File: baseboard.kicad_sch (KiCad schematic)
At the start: 27 parts, among them J10 AS7265X, J11 Conn_02x20_Odd_Even, J12 TFTLCD, J5 Screw_Terminal_01x02, J6 DCMI_CAMERA, J7 LCD_CHAR, J8 Conn_01x03, J9 Conn_01x03, U2 LM2676S-5, U3 AMS1117-3.3

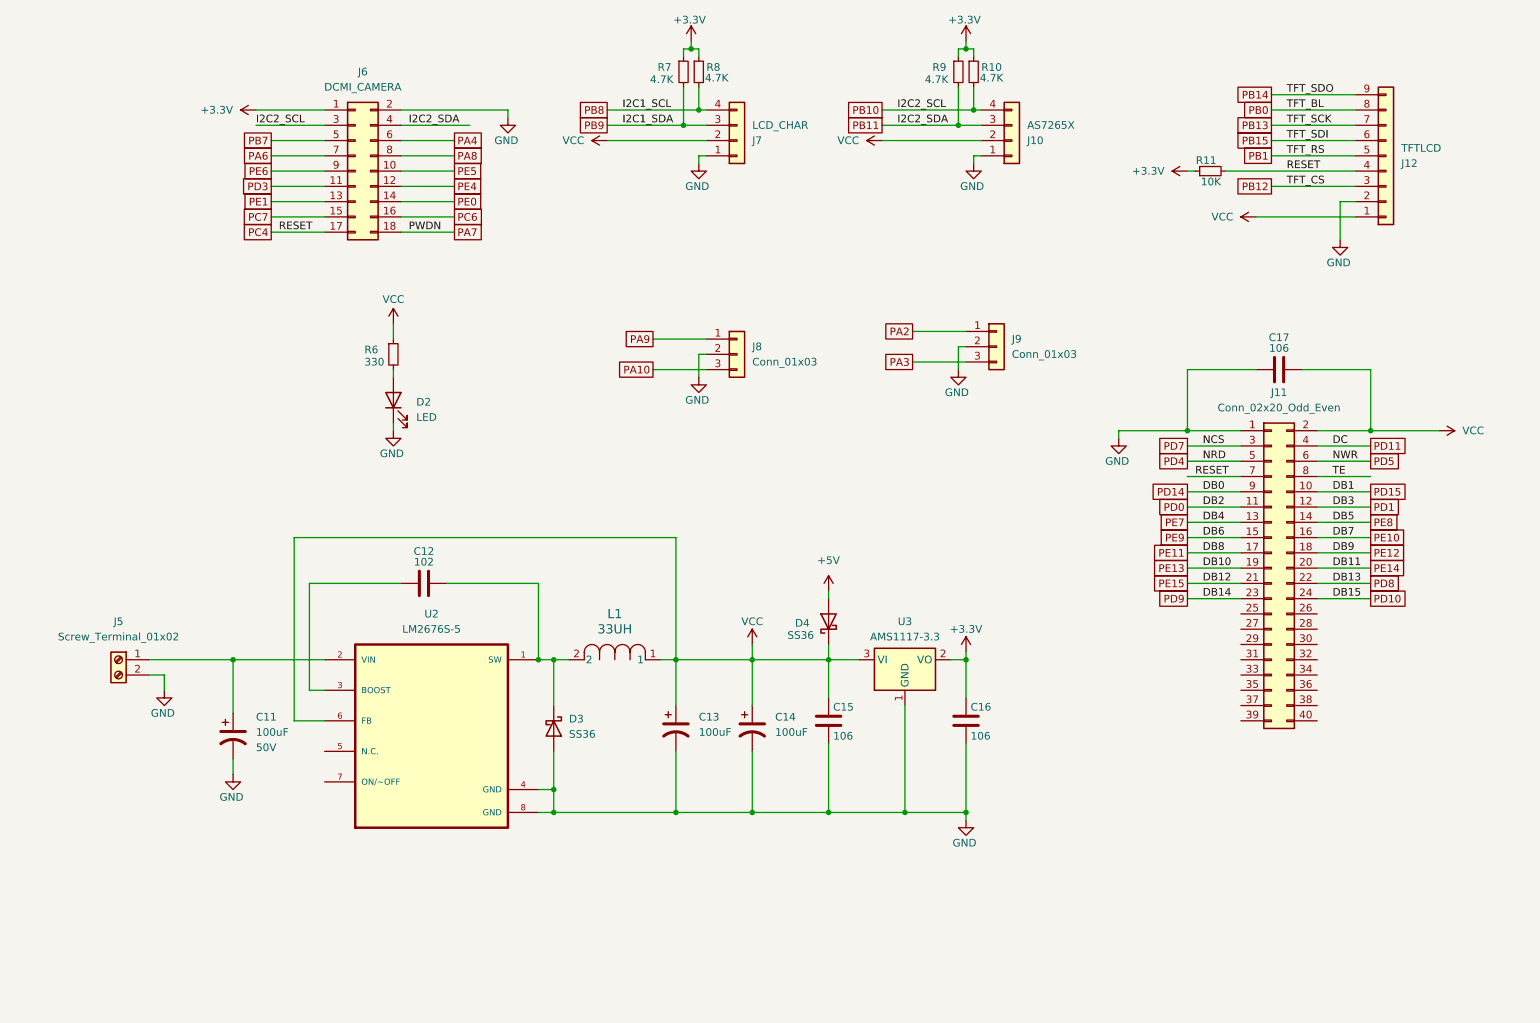
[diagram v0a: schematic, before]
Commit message: snapshot
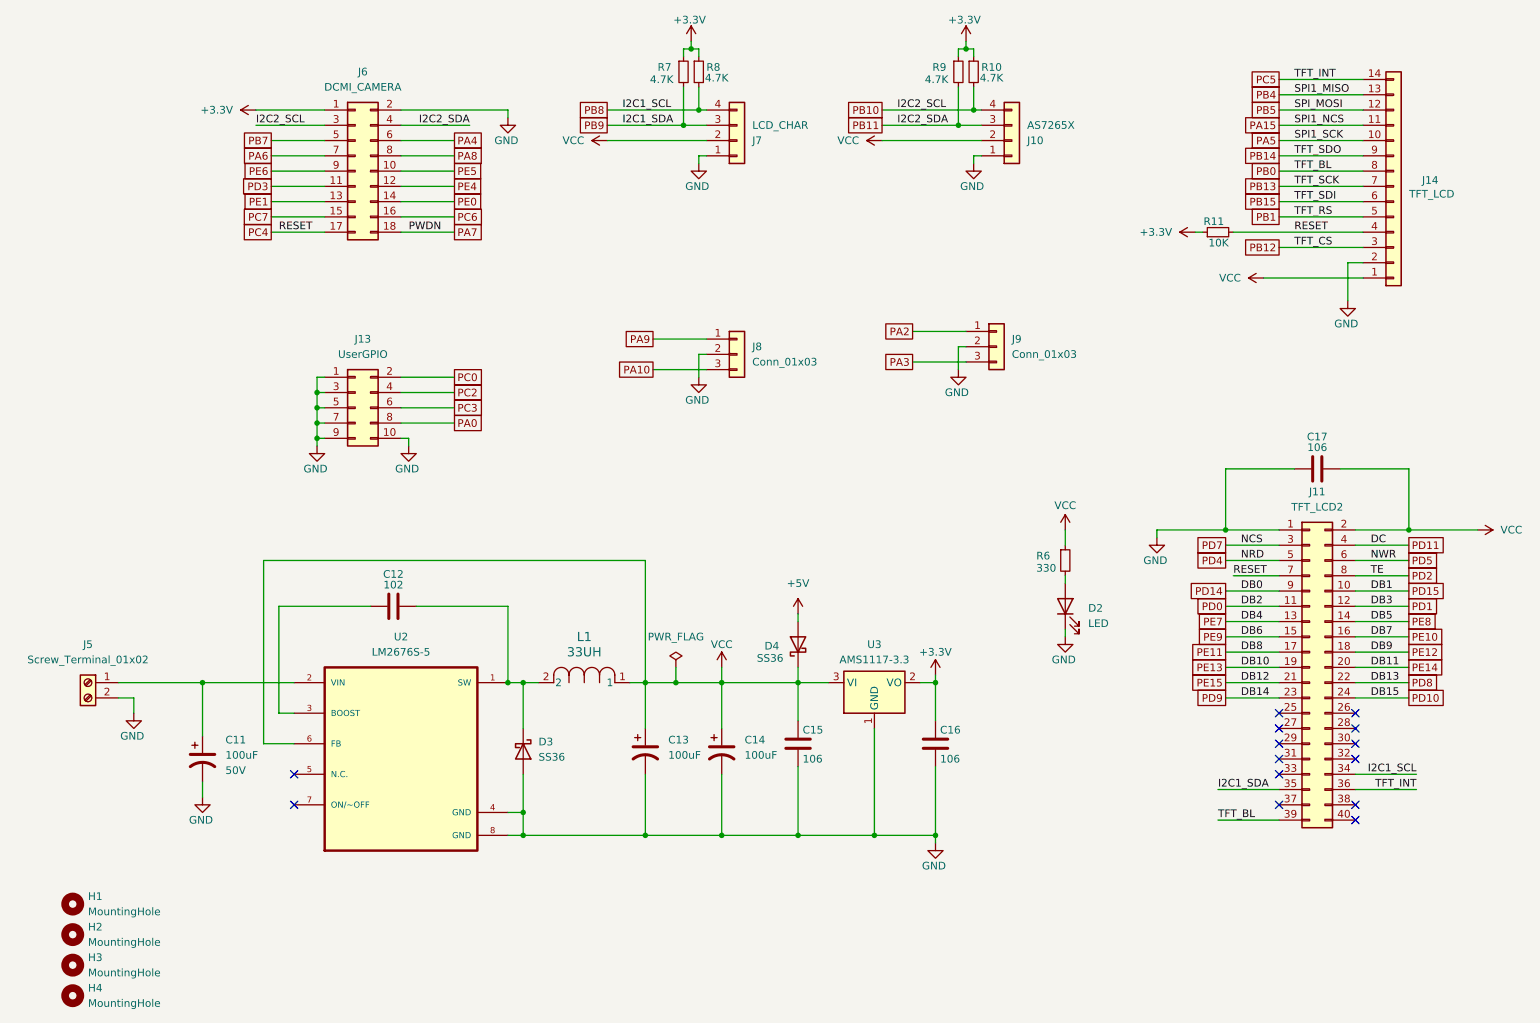
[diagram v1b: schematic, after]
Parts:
- removed J12: TFTLCD, Connector_PinHeader_2.54mm:PinHeader_1x09_P2.54mm_Vertical, symbol Connector_Generic:Conn_01x09
- added H1, H2, H3, H4: MountingHole, MountingHole:MountingHole_3.2mm_M3, symbol Mechanical:MountingHole
- added J13: UserGPIO, Connector_PinHeader_2.54mm:PinHeader_2x05_P2.54mm_Vertical, symbol Connector_Generic:Conn_02x05_Odd_Even
- added J14: TFT_LCD, Connector_PinHeader_2.54mm:PinHeader_1x14_P2.54mm_Vertical, symbol Connector_Generic:Conn_01x14
- J11: value Conn_02x20_Odd_Even -> TFT_LCD2
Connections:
- net GND: now also J13.1 (Pin_1), J13.10 (Pin_10), J13.3 (Pin_3), J13.5 (Pin_5), J13.7 (Pin_7), J13.9 (Pin_9), J14.2 (Pin_2)
- net PB0: now also J11.39 (Pin_39), J14.8 (Pin_8)
- net PB1: now also J14.5 (Pin_5)
- net PB12: now also J14.3 (Pin_3)
- net PB13: now also J14.7 (Pin_7)
- net PB14: now also J14.9 (Pin_9)
- net PB15: now also J14.6 (Pin_6)
- net PB8: now also J11.34 (Pin_34)
- net PB9: now also J11.35 (Pin_35)
- net PC4: now also J14.4 (Pin_4)
- net VCC: now also J14.1 (Pin_1)
- net PC5: now reaches J11.36 (Pin_36)
- net PC5: now also J14.14 (Pin_14)
- net TE renamed PD2
- new net PA0: J13.8 (Pin_8)
- new net PA15: J14.11 (Pin_11)
- new net PA5: J14.10 (Pin_10)
- new net PB4: J14.13 (Pin_13)
- new net PB5: J14.12 (Pin_12)
- new net PC0: J13.2 (Pin_2)
- new net PC2: J13.4 (Pin_4)
- new net PC3: J13.6 (Pin_6)
- no-connect marks 0 -> 14
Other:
- moved on the sheet: C11, C12, C13, C14, C15, C16, C17, D2, D3, D4, J11, J5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
